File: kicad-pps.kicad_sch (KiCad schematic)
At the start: 62 parts, among them J1 Conn_01x01_Pin, J10 Conn_01x01_Pin, J11 Conn_01x01_Pin, J12 Conn_01x01_Pin, J13 Conn_01x01_Pin, J14 Conn_01x01_Pin, J15 Conn_01x01_Pin, J16 Conn_01x01_Pin, J17 Conn_01x01_Pin, J18 Conn_01x01_Pin, J2 Conn_01x12_Pin, J3 Conn_01x01_Pin, J5 Conn_01x01_Pin, J6 Screw_Terminal_01x04, J7 AudioJack4, J8 AudioJack4, J9 AudioJack4, U1 HLK-5M05, U2 ESP32-C3-SuperMini, U3 MCP4131-xxxx-P, U4 MCP4131-xxxx-P, U5 MCP4131-xxxx-P, U6 LMV324, U7 LMV324

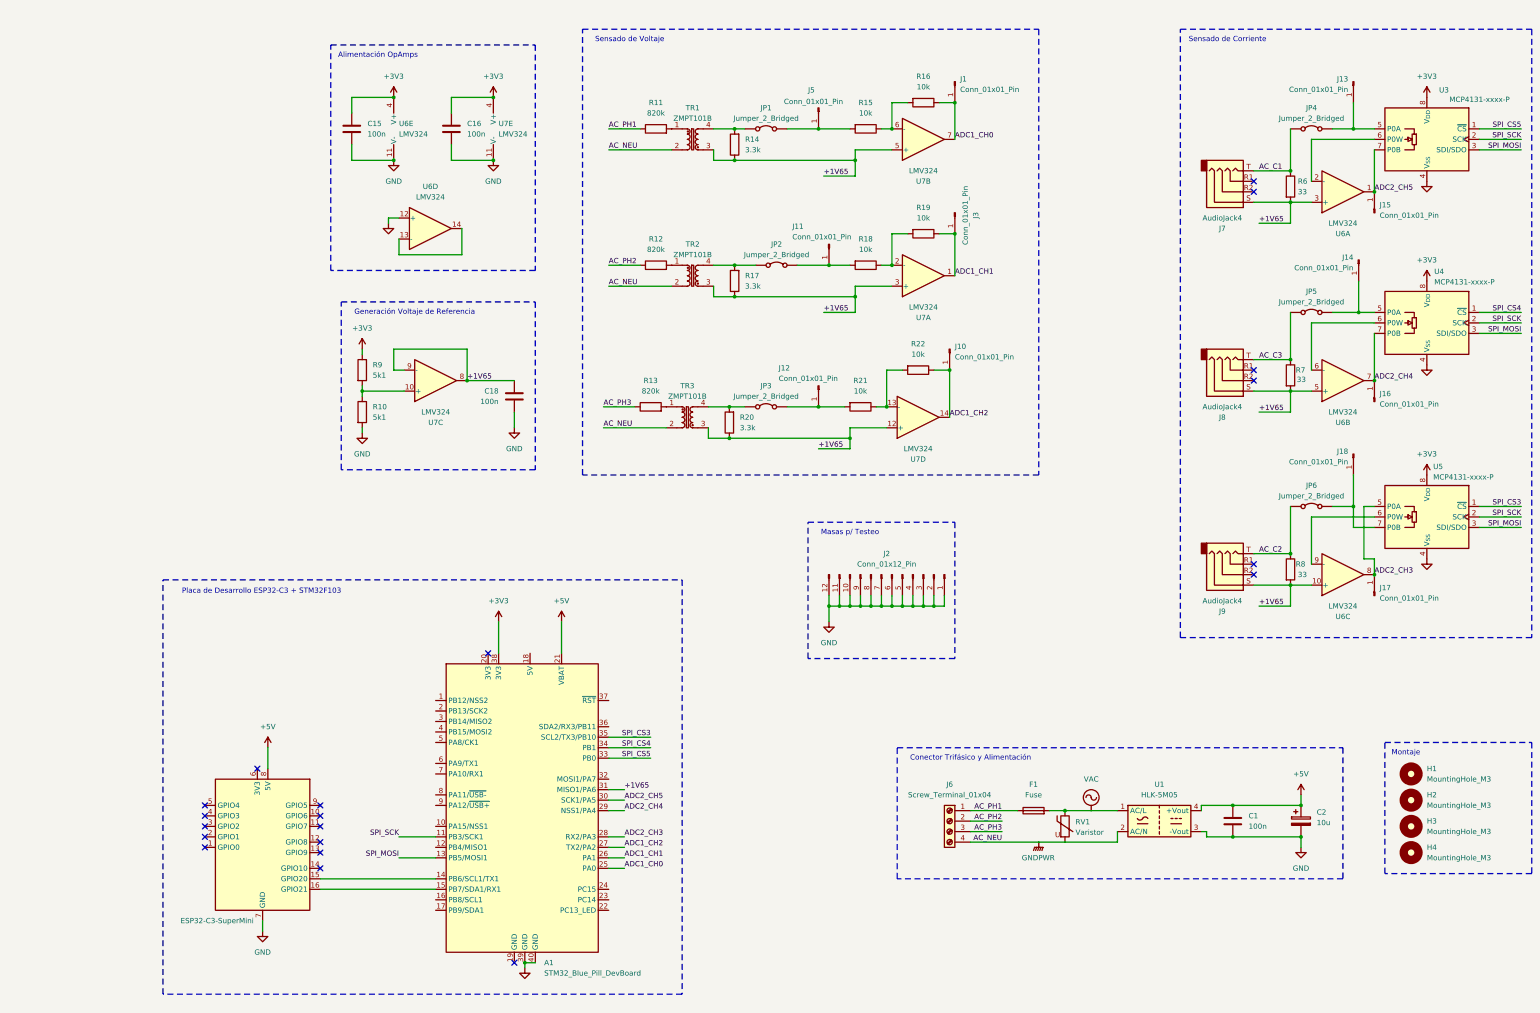
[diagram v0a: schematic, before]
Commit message: completo unicapa
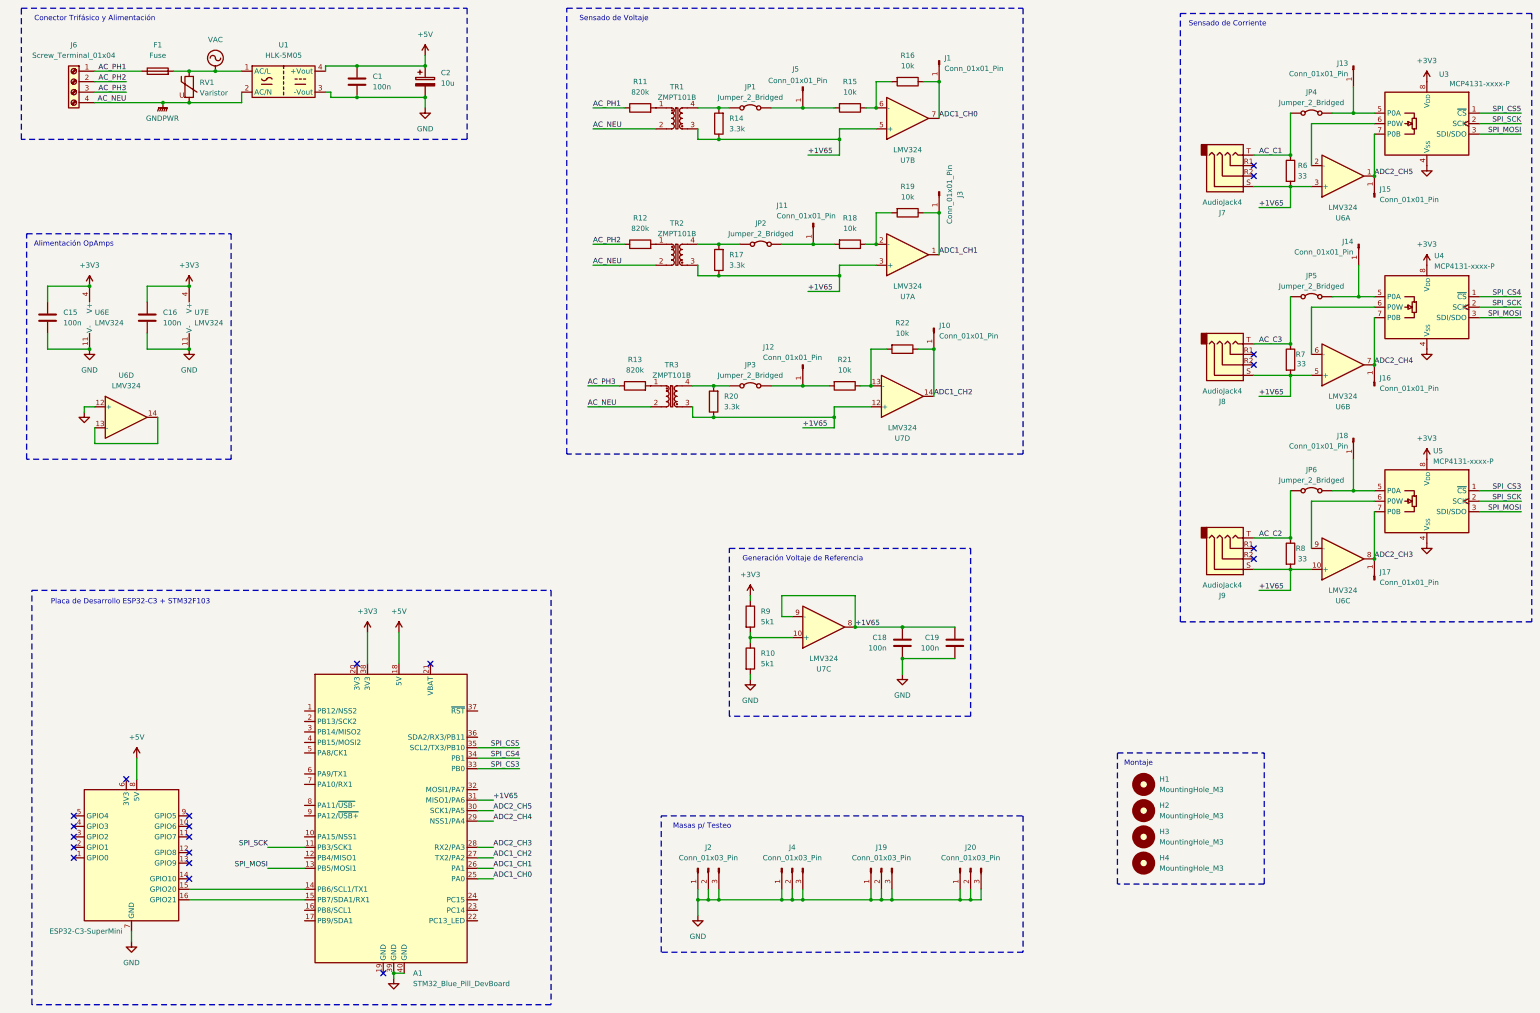
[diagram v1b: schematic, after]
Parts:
- removed J2: Conn_01x12_Pin, Connector_PinHeader_2.54mm:PinHeader_1x12_P2.54mm_Vertical, symbol Connector:Conn_01x12_Pin
- added C19: 100n, Capacitor_THT:CP_Radial_Tantal_D5.5mm_P2.50mm, symbol Device:C
- added J19, J2, J20, J4: Conn_01x03_Pin, Connector_PinHeader_2.54mm:PinHeader_1x03_P2.54mm_Vertical, symbol Connector:Conn_01x03_Pin
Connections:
- net +1V65: now also C19.1
- net +5V: now also A1.18 (5V); no longer A1.21 (VBAT)
- net ADC2_CH3: now also U5.7 (P0B); no longer U5.5 (P0A)
- net GND: now also C19.2, J19.1 (Pin_1), J19.2 (Pin_2), J19.3 (Pin_3), J2.1 (Pin_1), J2.2 (Pin_2), J2.3 (Pin_3), J20.1 (Pin_1), J20.2 (Pin_2), J20.3 (Pin_3), J4.1 (Pin_1), J4.2 (Pin_2), J4.3 (Pin_3)
- net SPI_CS3: now also A1.33 (PB0); no longer A1.35 (SCL2/TX3/PB10)
- net SPI_CS5: now also A1.35 (SCL2/TX3/PB10); no longer A1.33 (PB0)
- net at J18.1 (Pin_1), JP6.2 (B): now also U5.5 (P0A); no longer U5.7 (P0B)
- no-connect marks 20 -> 21
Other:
- moved on the sheet: A1, C1, C15, C16, C18, C2, F1, H1, H2, H3, H4, J1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
